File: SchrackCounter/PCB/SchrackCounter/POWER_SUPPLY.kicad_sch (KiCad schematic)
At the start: 14 parts, among them IC1 TPS565242DRLR, SW1 SW_DPDT_x2

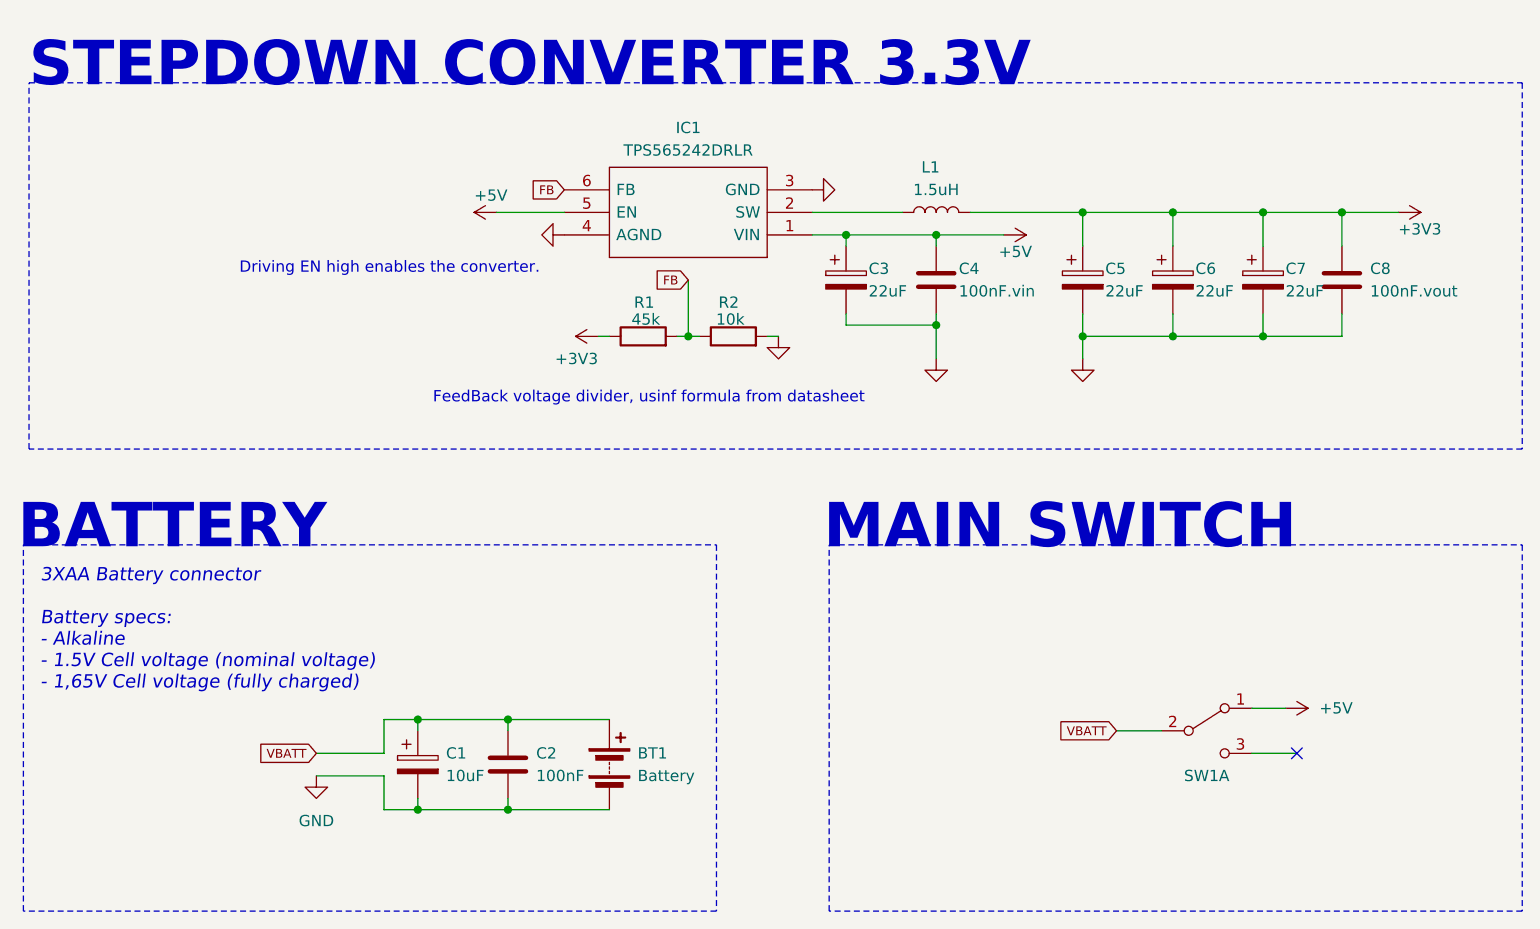
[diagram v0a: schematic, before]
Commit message: sleep, overated imo
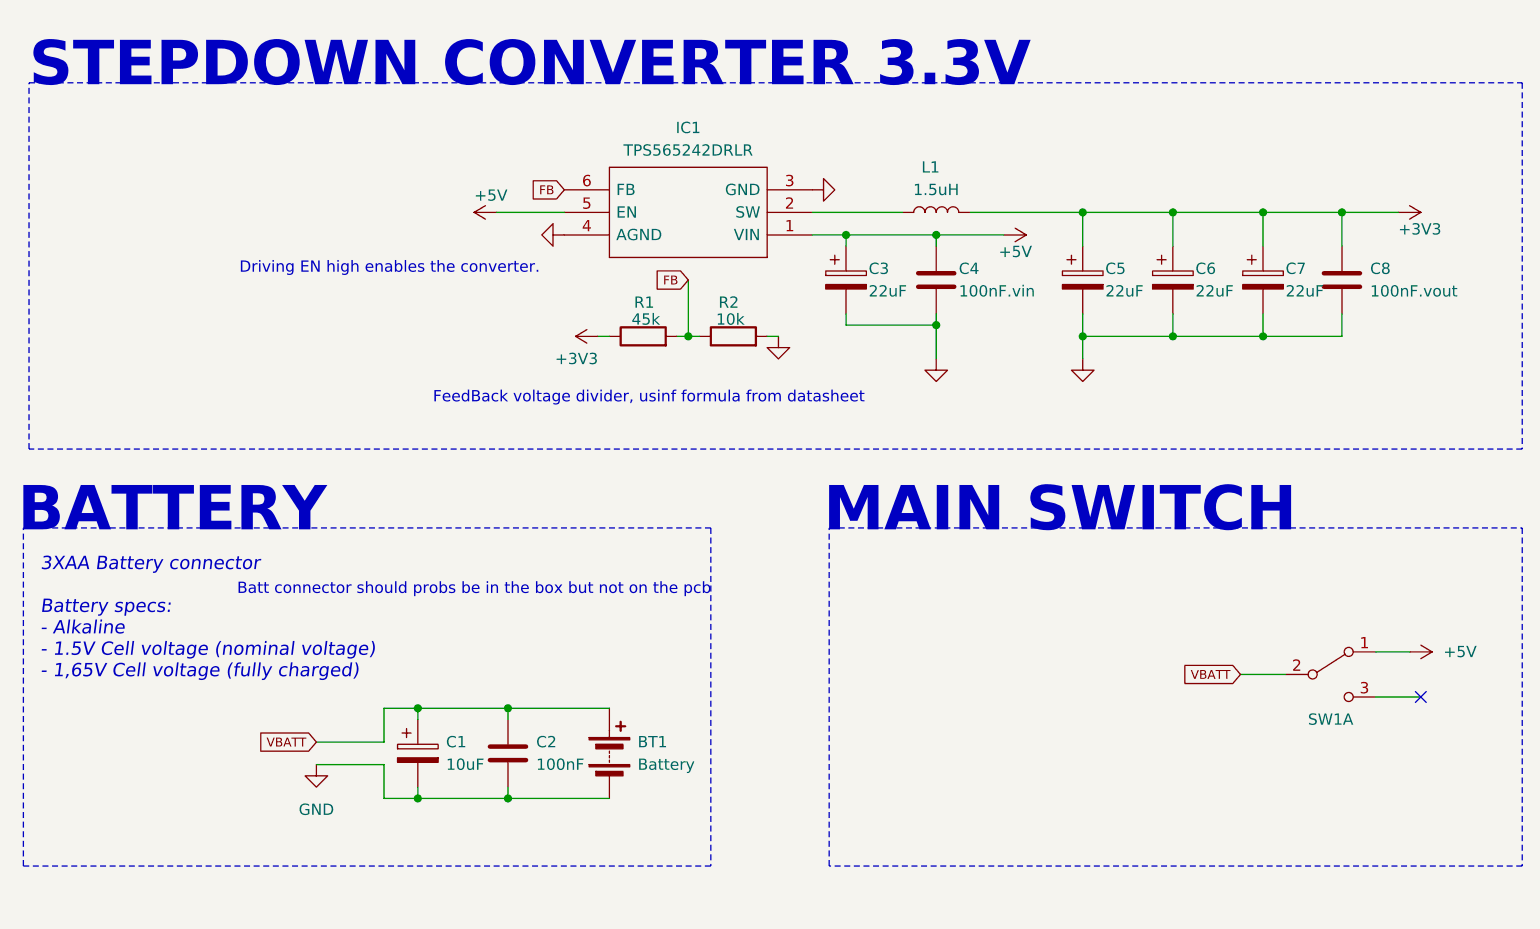
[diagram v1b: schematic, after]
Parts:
- BT1: footprint Battery:BatteryHolder_Keystone_2462_2xAA - no holes -> Connector_Samtec_HPM_THT:Samtec_HPM-02-01-x-S_Straight_1x02_Pitch5.08mm
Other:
- note added: "Batt connector should probs be in the box but not on the pcb"
- moved on the sheet: BT1, C1, C2, SW1A
